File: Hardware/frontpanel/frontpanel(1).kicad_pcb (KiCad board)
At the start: 2 copper layers, 91.3 x 128.5 mm, 42 parts

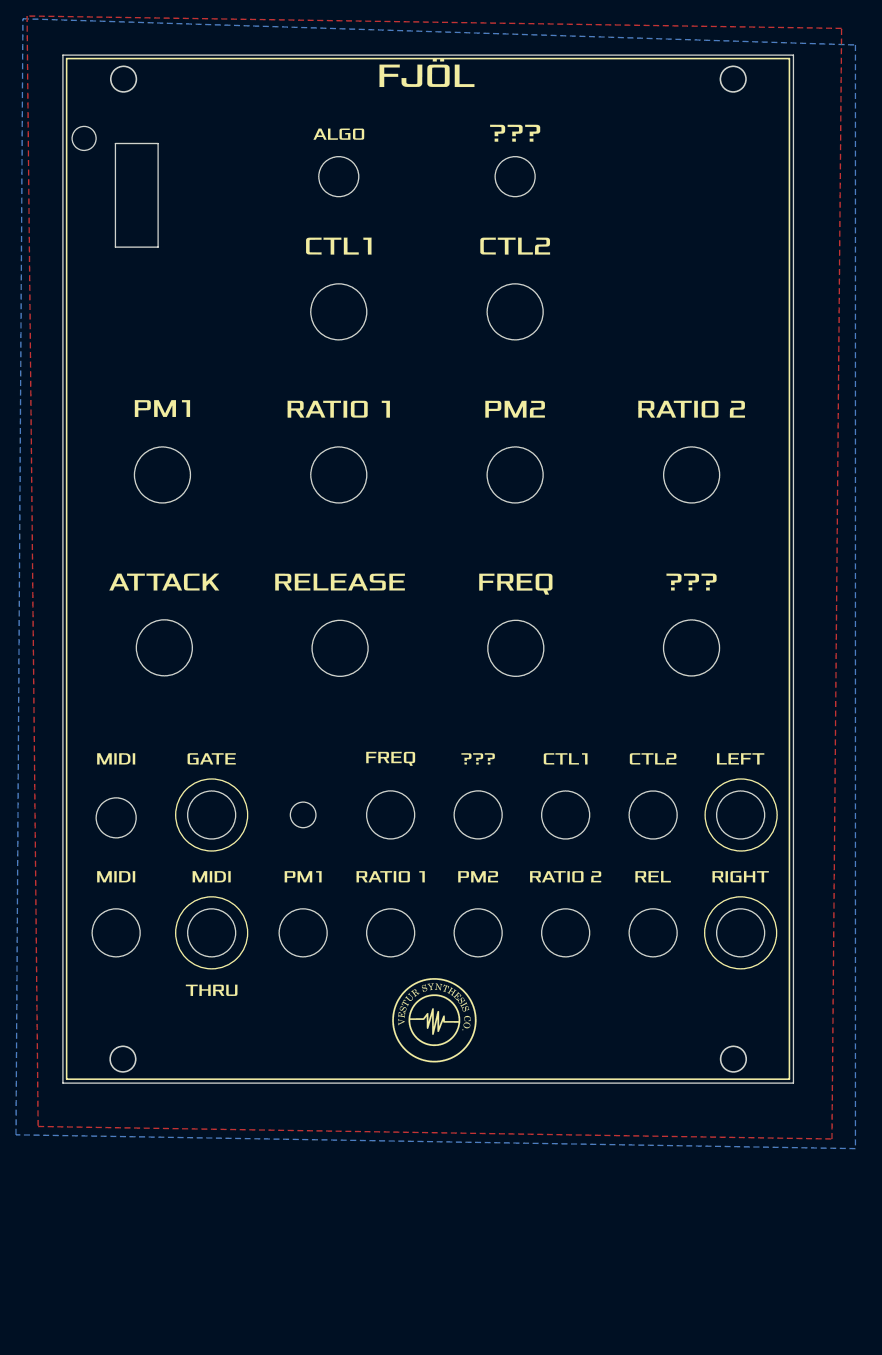
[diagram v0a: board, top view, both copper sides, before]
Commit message: update
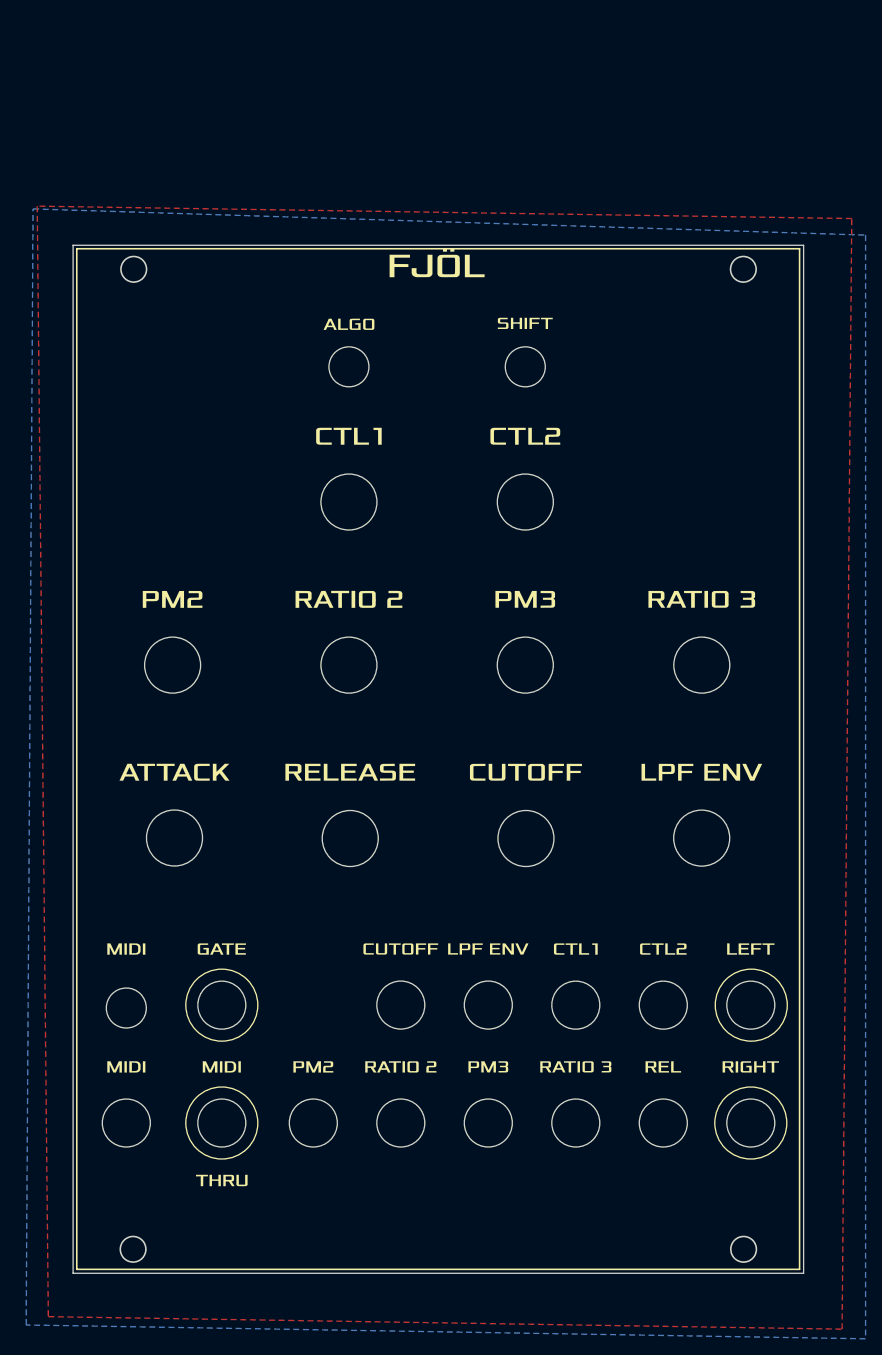
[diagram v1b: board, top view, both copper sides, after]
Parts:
- removed the G*** at (170.0, 76.4)
- removed the G*** at (137.9, 131.1)
- removed the G*** at (121.4, 113.2)
- removed the G*** at (132.4, 113.2)
- removed the G*** at (132.4, 98.5)
- removed the G*** at (103.8, 54.7)
- removed the G*** at (158.9, 45.6)
- removed the G*** at (158.9, 34.7)
- removed the G*** at (125.9, 54.8)
- removed the G*** at (158.9, 51.0)
- removed the G*** at (158.9, 40.2)
- removed the G*** at (148.0, 76.7)
- added G***: LOGO, vestur-logo:cutoff, F.Cu at (149.3, 100.2)
- added G***: LOGO, vestur-logo:decay, F.Cu at (116.1, 69.4)
- added G***: LOGO, vestur-logo:cutoff-small, F.Cu at (133.6, 122.3)
- added G***: LOGO, vestur-logo:filt-env-knob, F.Cu at (171.2, 100.2)
- added G***: LOGO, vestur-logo:ratio3, F.Cu at (171.2, 78.6)
- added G***: LOGO, vestur-logo:pm3-small, F.Cu at (144.6, 137.0)
- added G***: LOGO, vestur-logo:glide, F.Cu at (116.1, 74.9)
- added G***: LOGO, vestur-logo:pm3, F.Cu at (149.2, 78.6)
- added G***: LOGO, vestur-logo:ratio3-small, F.Cu at (155.5, 137.0)
- added G***: LOGO, vestur-logo:decay-mirror, B.Cu at (116.1, 69.4)
- added G*** (x2): LOGO, vestur-logo:feedback-mirror, B.Cu at (160.2, 69.4)
- added G***: LOGO, vestur-logo:feedback2-mirror, B.Cu at (160.2, 74.8)
- added G***: LOGO, vestur-logo:det2-mirror, B.Cu at (160.2, 58.4)
- added G***: LOGO, vestur-logo:det3-mirror, B.Cu at (160.2, 63.9)
- added G***: LOGO, vestur-logo:glide-mirror, B.Cu at (116.1, 74.9)
- G***: footprint vestur-logo:???-small -> vestur-logo:filt-env-jack
- G***: footprint vestur-logo:pwm-solderm -> vestur-logo:feedback2
- G***: footprint vestur-logo:saw-solderm -> vestur-logo:det2
- G***: footprint vestur-logo:det-solderm -> vestur-logo:det3
- G***: footprint vestur-logo:square-solderm -> vestur-logo:feedback
- G***: footprint vestur-logo:??? -> vestur-logo:shift
- moved G*** 49.0 mm to (127.1, 78.6)
- moved G*** 49.0 mm to (105.1, 78.6)
- moved G*** 31.5 mm to (122.7, 137.0)
- moved G*** 31.5 mm to (133.6, 137.0)
- moved G*** 23.8 mm to (99.3, 137.0)
- moved G*** 23.8 mm to (111.2, 137.0)
- moved G*** 23.8 mm to (127.3, 100.2)
- moved G*** 23.8 mm to (105.3, 100.2)
- moved G*** 23.8 mm to (177.4, 137.0)
- moved G*** 23.8 mm to (166.4, 137.0)
- moved G*** 23.8 mm to (138.2, 36.5)
- moved G*** 23.8 mm to (116.1, 58.5) (x2)
- moved G*** 23.8 mm to (160.2, 58.4)
- moved G*** 23.8 mm to (127.1, 58.2)
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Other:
- outline, holes or cut-outs redrawn
